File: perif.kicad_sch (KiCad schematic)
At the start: 31 parts, among them J10 Conn_01x04, J12 Conn_01x10, J13 Conn_01x10, J14 Conn_01x10, J15 Screw_Terminal_01x02, J18 Screw_Terminal_01x02, J20 Conn_01x10, J4 Conn_02x02_Odd_Even, J6 Conn_01x04, J9 Conn_01x05, U2 TCAN332G, U3 MCP2518FD-xQBB, U4 PCA9685BS, U5 SN74LVC8T245PWR, U6 SN74LVC8T245PWR, Y1 Crystal

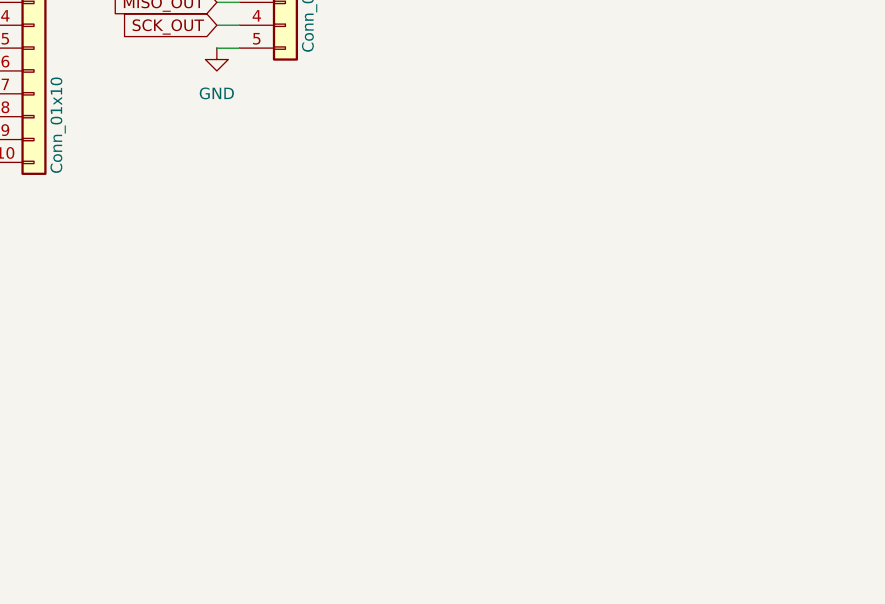
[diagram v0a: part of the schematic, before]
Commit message: Implementing just so much stuff. RP2350B on board, new sensors, PSU magic, buncha stuff
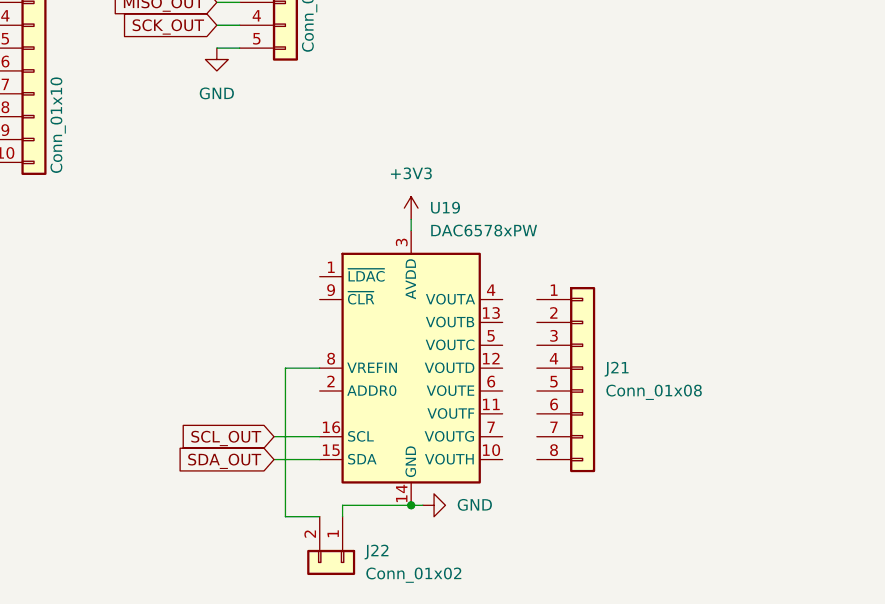
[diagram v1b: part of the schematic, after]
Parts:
- added J21: Conn_01x08, symbol Connector_Generic:Conn_01x08
- added J22: Conn_01x02, Connector_JST:JST_PH_B2B-PH-K_1x02_P2.00mm_Vertical, symbol Connector_Generic:Conn_01x02
- added U19: DAC6578xPW, Package_SO:TSSOP-16_4.4x5mm_P0.65mm, symbol Analog_DAC:DAC6578xPW
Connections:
- net +3V3: now also U19.3 (AVDD)
- net GND: now also J22.1 (Pin_1), U19.14 (GND)
- net SCL_OUT: now also U19.16 (SCL)
- net SDA_OUT: now also U19.15 (SDA)
- new net: J22.2 (Pin_2), U19.8 (VREFIN)

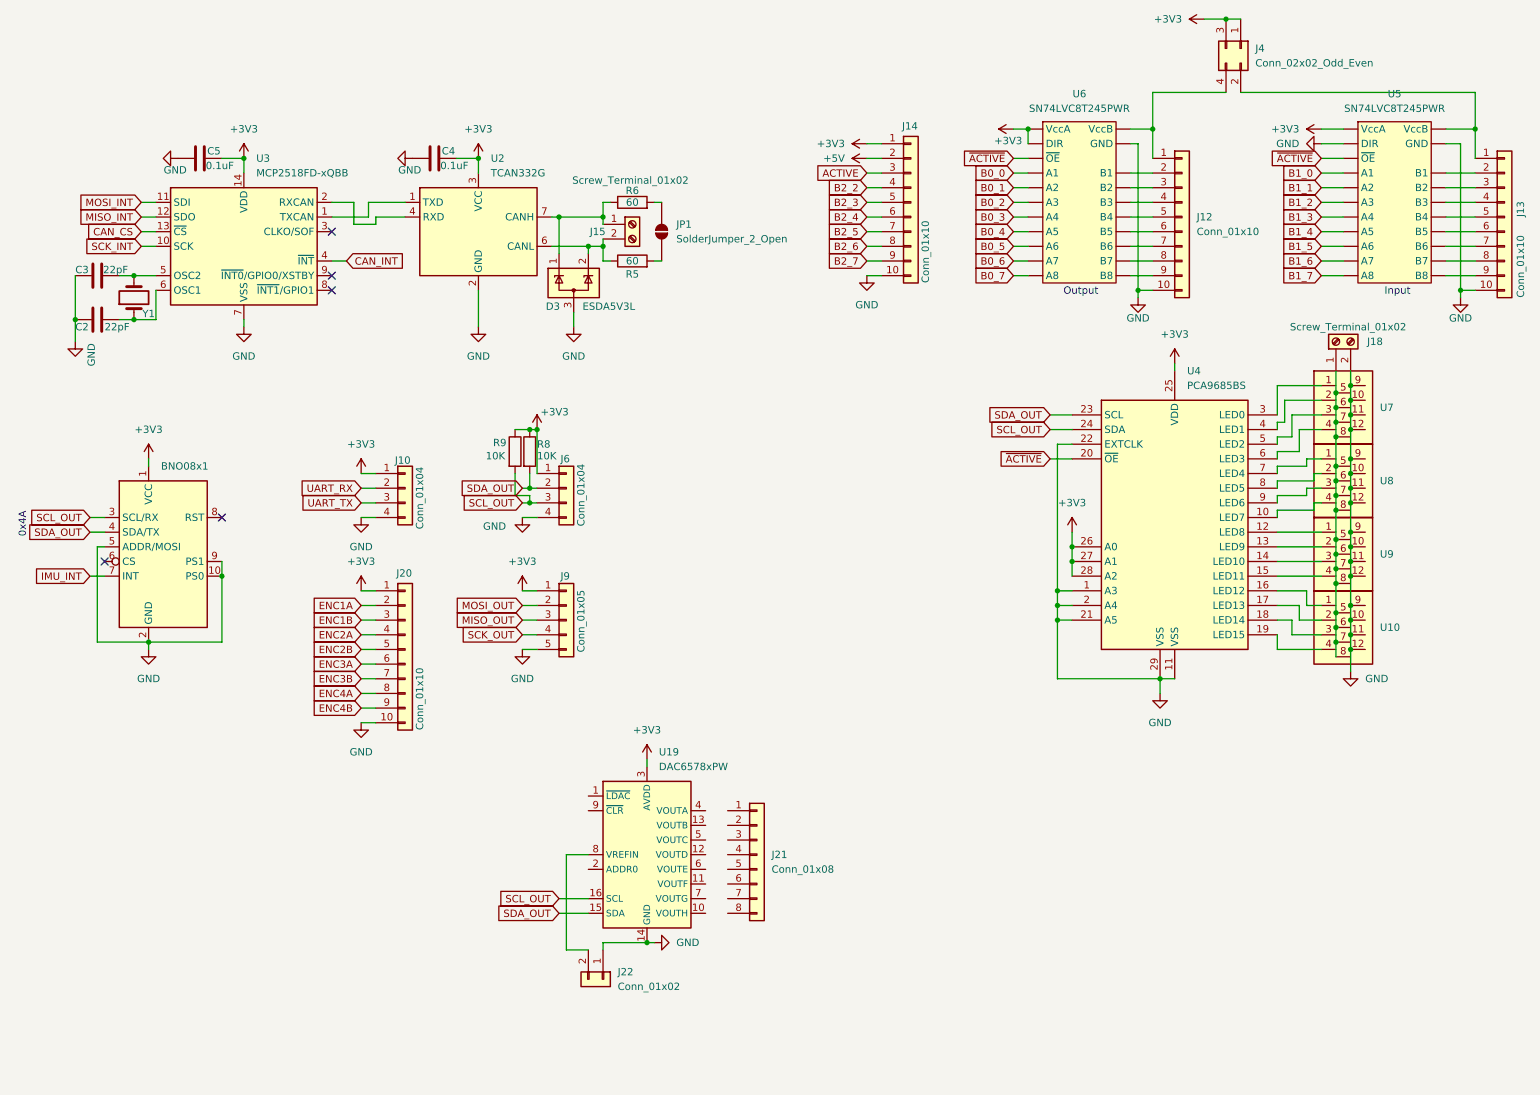
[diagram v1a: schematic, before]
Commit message: Switched back to 2350A, rewired FPGA pins, maybe added some stuff? Idk.
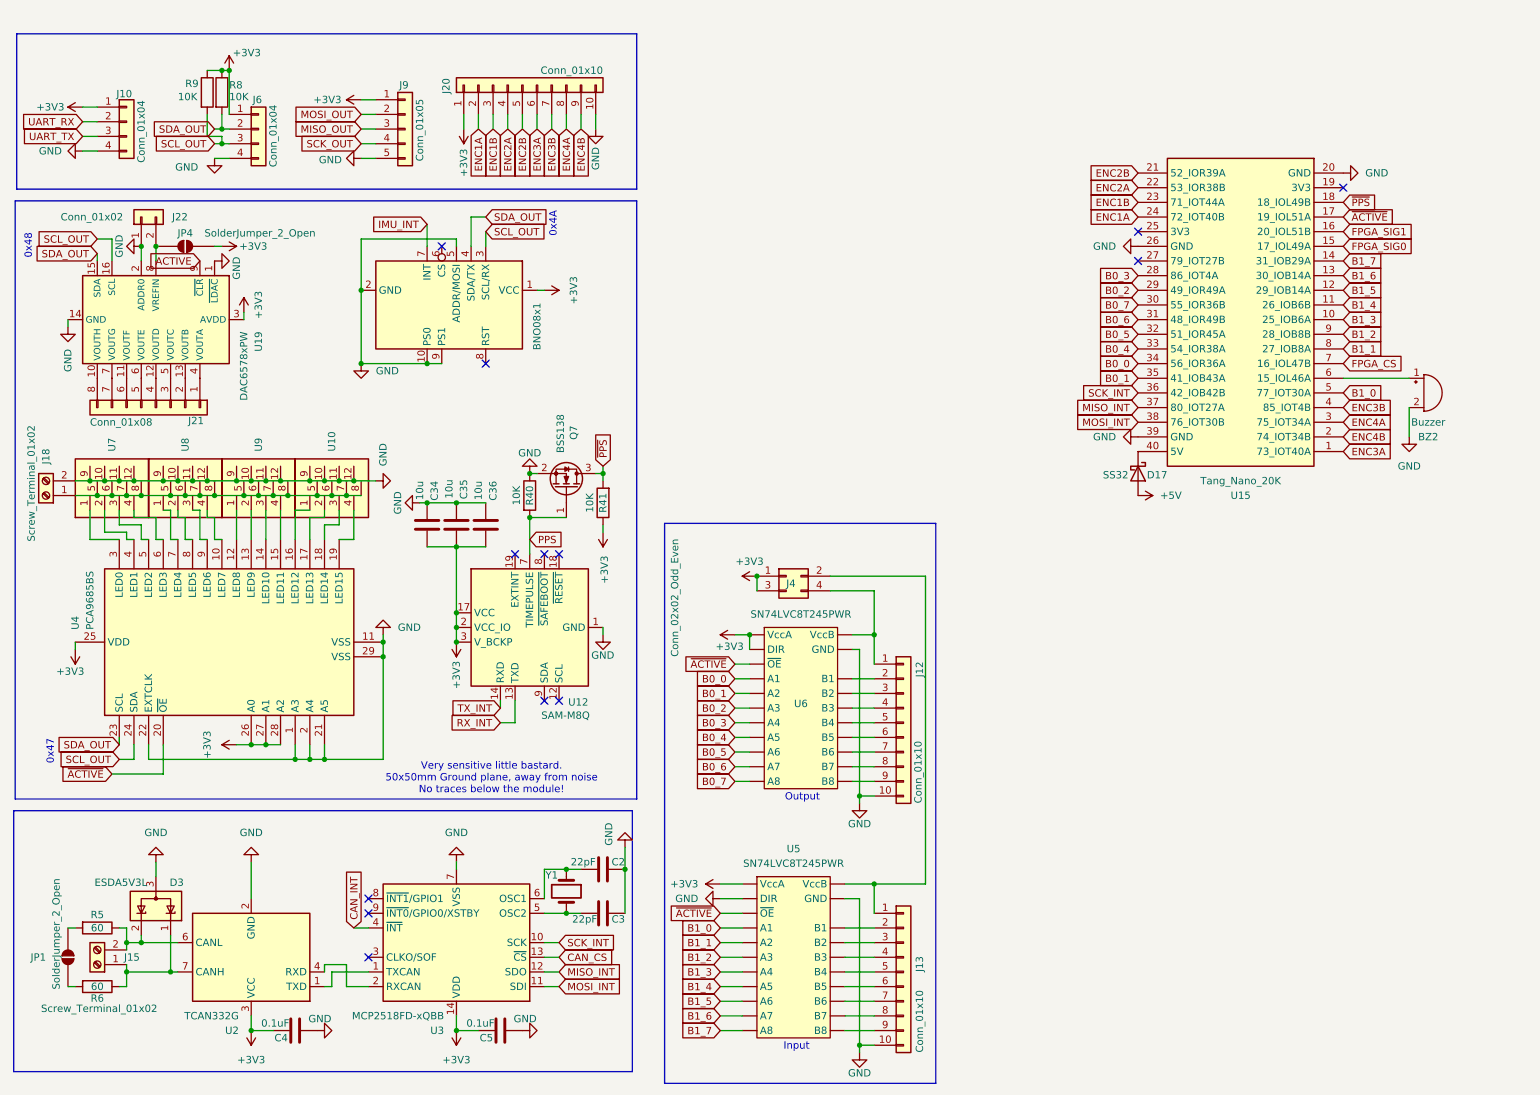
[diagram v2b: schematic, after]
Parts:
- removed J14: Conn_01x10, Connector_JST:JST_GH_BM10B-GHS-TBT_1x10-1MP_P1.25mm_Vertical, symbol Connector_Generic:Conn_01x10
- added BZ2: Buzzer, Buzzer_Beeper:Buzzer_12x9.5RM7.6, symbol Device:Buzzer
- added C34, C35, C36: 10u, Capacitor_SMD:C_0402_1005Metric, symbol Device:C
- added D17: SS32, Diode_SMD:D_SMA, symbol Diode:SS32
- added JP4: SolderJumper_2_Open, Jumper:SolderJumper-2_P1.3mm_Open_TrianglePad1.0x1.5mm, symbol Jumper:SolderJumper_2_Open
- added Q7: BSS138, Package_TO_SOT_SMD:SOT-23, symbol Transistor_FET:BSS138
- added R40, R41: 10K, Resistor_SMD:R_0603_1608Metric_Pad0.98x0.95mm_HandSolder, symbol Device:R
- added U12: SAM-M8Q, RF_GPS:ublox_SAM-M8Q, symbol RF_GPS:SAM-M8Q
- added U15: Tang_Nano_20K, 0my_project:DIP-40_TangNano20K, symbol 0my_project:Tang_Nano_20K
- C2, C3, C4, C5: footprint Capacitor_SMD:C_0201_0603Metric_Pad0.64x0.40mm_HandSolder -> Capacitor_SMD:C_0402_1005Metric_Pad0.74x0.62mm_HandSolder
- J21: footprint (none) -> Connector_JST:JST_GH_BM08B-GHS-TBT_1x08-1MP_P1.25mm_Vertical
- R5: footprint Resistor_SMD:R_1812_4532Metric_Pad1.30x3.40mm_HandSolder -> Resistor_SMD:R_1812_4532Metric
- Y1: value Crystal -> 20mHz; footprint Crystal:Crystal_SMD_5032-2Pin_5.0x3.2mm -> Inductor_SMD:L_1008_2520Metric_Pad1.43x2.20mm_HandSolder
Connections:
- net +3V3: now also C34.1, C35.1, C36.1, JP4.1 (A), R41.1, U12.17 (VCC), U12.2 (VCC_IO), U12.3 (V_BCKP)
- net +5V: now also D17.2 (A)
- net ACTIVE: now also U19.9 (~{CLR})
- net B0_0: now also U15.34 (56_IOR36A)
- net B0_1: now also U15.35 (41_IOB43A)
- net B0_2: now also U15.29 (49_IOR49A)
- net B0_3: now also U15.28 (86_IOT4A)
- net B0_4: now also U15.33 (54_IOR38A)
- net B0_5: now also U15.32 (51_IOR45A)
- net B0_6: now also U15.31 (48_IOR49B)
- net B0_7: now also U15.30 (55_IOR36B)
- net B1_0: now also U15.5 (77_IOT30A)
- net B1_1: now also U15.8 (27_IOB8A)
- net B1_2: now also U15.9 (28_IOB8B)
- net B1_3: now also U15.10 (25_IOB6A)
- net B1_4: now also U15.11 (26_IOB6B)
- net B1_5: now also U15.12 (29_IOB14A)
- net B1_6: now also U15.13 (30_IOB14A)
- net B1_7: now also U15.14 (31_IOB29A)
- net ENC1A: now also U15.24 (72_IOT40B)
- net ENC1B: now also U15.23 (71_IOT44A)
- net ENC2A: now also U15.22 (53_IOR38B)
- net ENC2B: now also U15.21 (52_IOR39A)
- net ENC3A: now also U15.1 (73_IOT40A)
- net ENC3B: now also U15.4 (85_IOT4B)
- net ENC4A: now also U15.3 (75_IOT34A)
- net ENC4B: now also U15.2 (74_IOT34B)
- net GND: now also U19.1 (~{LDAC}), U19.2 (ADDR0), BZ2.2 (-), C34.2, C35.2, C36.2, Q7.2 (S), R40.1, U12.1 (GND), U12.10 (GND), U12.11 (GND), U12.15 (GND), U12.16 (GND), U12.20 (GND), U12.4 (GND), U12.5 (GND), U12.6 (GND), U15.20 (GND), U15.26 (GND), U15.39 (GND)
- net MISO_INT: now also U15.37 (80_IOT27A)
- net MOSI_INT: now also U15.38 (76_IOT30B)
- net SCK_INT: now also U15.36 (42_IOB42B)
- net ~{ACTIVE}: now also U15.17 (19_IOL51A)
- net at J22.2 (Pin_2), U19.8 (VREFIN): now also JP4.2 (B)
- net at J21.1 (Pin_1): now also U19.4 (VOUTA)
- net at J21.2 (Pin_2): now also U19.13 (VOUTB)
- net at J21.3 (Pin_3): now also U19.5 (VOUTC)
- net at J21.4 (Pin_4): now also U19.12 (VOUTD)
- net at J21.5 (Pin_5): now also U19.6 (VOUTE)
- net at J21.6 (Pin_6): now also U19.11 (VOUTF)
- net at J21.7 (Pin_7): now also U19.7 (VOUTG)
- net at J21.8 (Pin_8): now also U19.10 (VOUTH)
- new net: D17.1 (K), U15.40 (5V)
- new net: BZ2.1 (+), U15.6 (15_IOL46A)
- new net FPGA_CS: U15.7 (16_IOL47B)
- new net FPGA_SIG0: U15.15 (17_IOL49A)
- new net FPGA_SIG1: U15.16 (20_IOL51B)
- new net PPS: Q7.1 (G), R40.2, U12.7 (TIMEPULSE)
- new net RX_INT: U12.13 (TXD)
- new net TX_INT: U12.14 (RXD)
- new net ~{PPS}: Q7.3 (D), R41.2, U15.18 (18_IOL49B)
- no-connect marks 5 -> 13
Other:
- note added: "0x47"
- note added: "0x48"
- note added: "Very sensitive little bastard. 50x50mm Ground plane, away from noise No traces below the module!"
- moved on the sheet: BNO08x1, C2, C3, C4, C5, D3, J10, J12, J13, J15, J18, J20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
